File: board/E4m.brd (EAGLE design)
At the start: 49.4 x 100.1 mm, 76 parts, among them IC1 MCP23017SS, Q1 IRL540, Q2 IRL540, Q3 IRL540

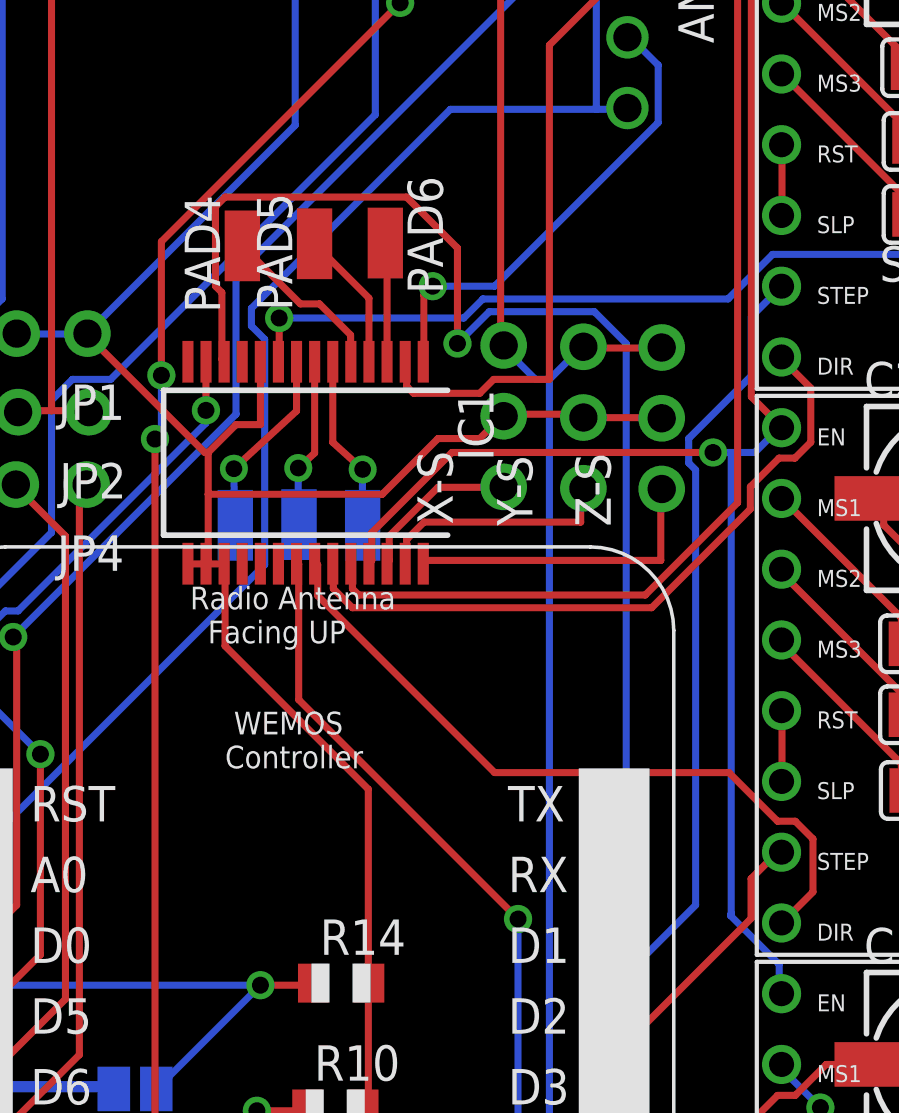
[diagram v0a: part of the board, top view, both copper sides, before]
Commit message: clean clean clean
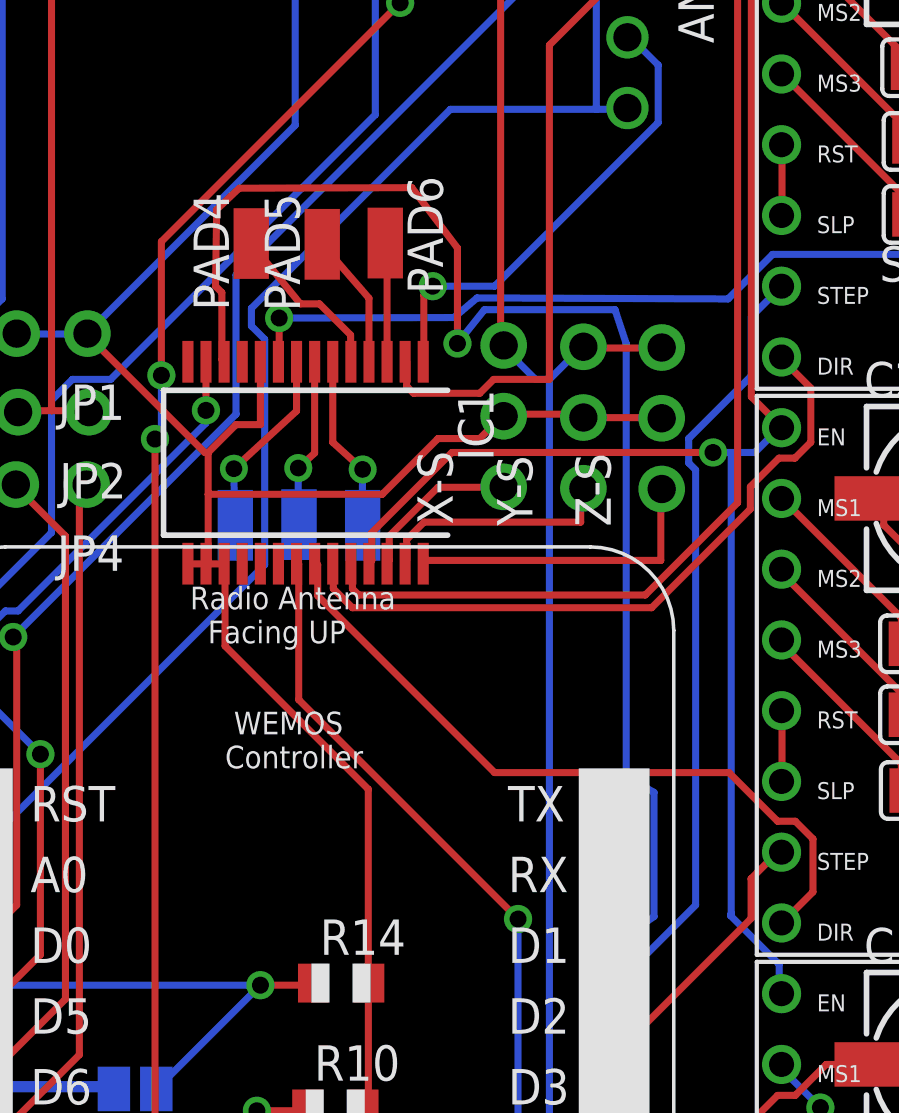
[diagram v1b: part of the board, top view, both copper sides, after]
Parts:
- moved PAD4 0.33 mm to (13.2, 47.3)
- moved PAD5 0.28 mm to (15.7, 47.2)
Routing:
- net SCL: track 48.0 -> 49.5 mm
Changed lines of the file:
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@@
 <element name="PAD2" library="wirepad" package="SMD1,27-2,54" value="WIREPADSMD1,27-254" x="17.1704" y="37.1348" rot="MR0"/>
 <element name="PAD3" library="wirepad" package="SMD1,27-2,54" value="WIREPADSMD1,27-254" x="14.8844" y="37.1602" rot="MR0"/>
-<element name="PAD4" library="wirepad" package="SMD1,27-2,54" value="WIREPADSMD1,27-254" x="12.8524" y="47.1678"/>
-<element name="PAD5" library="wirepad" package="SMD1,27-2,54" value="WIREPADSMD1,27-254" x="15.4432" y="47.244"/>
+<element name="PAD4" library="wirepad" package="SMD1,27-2,54" value="WIREPADSMD1,27-254" x="13.1699" y="47.251621875"/>
+<element name="PAD5" library="wirepad" package="SMD1,27-2,54" value="WIREPADSMD1,27-254" x="15.720059375" y="47.223678125"/>
 <element name="PAD6" library="wirepad" package="SMD1,27-2,54" value="WIREPADSMD1,27-254" x="17.9832" y="47.2694" rot="R180"/>
 <element name="JP3" library="adafruit" package="1X01-CLEANBIG" value="" x="24.0284" y="85.8266"/>
@@
 <wire x1="16.7386" y1="43.9674" x2="15.621" y2="45.085" width="0.254" layer="1"/>
 <wire x1="15.621" y1="45.085" x2="14.9352" y2="45.085" width="0.254" layer="1"/>
-<wire x1="14.9352" y1="45.085" x2="12.8524" y2="47.1678" width="0.254" layer="1"/>
+<wire x1="14.9352" y1="45.085" x2="13.1699" y2="47.251621875" width="0.254" layer="1"/>
 </signal>
 <signal name="N$26" class="3">
 <contactref element="IC1" pad="4"/>
 <contactref element="PAD5" pad="1"/>
-<wire x1="15.4432" y1="47.244" x2="17.397" y2="45.2902" width="0.254" layer="1"/>
+<wire x1="15.720059375" y1="47.223678125" x2="17.397" y2="45.2902" width="0.254" layer="1"/>
 <wire x1="17.397" y1="45.2902" x2="17.397" y2="43.006" width="0.254" layer="1"/>
 </signal>
@@
 <wire x1="12.1158" y1="45.4914" x2="12.1158" y2="43.0911" width="0.254" layer="1"/>
 <wire x1="11.8872" y1="45.72" x2="12.1158" y2="45.4914" width="0.254" layer="1"/>
-<wire x1="11.8872" y1="48.5775" x2="11.8872" y2="45.72" width="0.254" layer="1"/>
-<wire x1="12.2301" y1="48.9204" x2="11.8872" y2="48.5775" width="0.254" layer="1"/>
-<wire x1="18.7452" y1="48.9204" x2="12.2301" y2="48.9204" width="0.254" layer="1"/>
-<wire x1="20.574" y1="47.0916" x2="18.7452" y2="48.9204" width="0.254" layer="1"/>
+<wire x1="11.93038125" y1="48.4733625" x2="11.8872" y2="45.72" width="0.254" layer="1"/>
+<wire x1="12.7381" y1="49.2379" x2="11.93038125" y2="48.4733625" width="0.254" layer="1"/>
+<wire x1="18.9357" y1="49.25821875" x2="12.7381" y2="49.2379" width="0.254" layer="1"/>
+<wire x1="20.574" y1="47.0916" x2="18.9357" y2="49.25821875" width="0.254" layer="1"/>
 <wire x1="20.574" y1="43.6626" x2="20.574" y2="47.0916" width="0.254" layer="1"/>
-<wire x1="21.717" y1="44.8056" x2="20.574" y2="43.6626" width="0.254" layer="16"/>
-<wire x1="25.4889" y1="44.8056" x2="21.717" y2="44.8056" width="0.254" layer="16"/>
-<wire x1="26.6319" y1="43.6626" x2="25.4889" y2="44.8056" width="0.254" layer="16"/>
+<wire x1="21.541740625" y1="44.876721875" x2="20.574" y2="43.6626" width="0.254" layer="16"/>
+<wire x1="26.23058125" y1="44.87671875" x2="21.541740625" y2="44.876721875" width="0.254" layer="16"/>
+<wire x1="26.6319" y1="43.6626" x2="26.23058125" y2="44.87671875" width="0.254" layer="16"/>
 <wire x1="26.6319" y1="28.1178" x2="26.6319" y2="43.6626" width="0.254" layer="16"/>
-<wire x1="27.2034" y1="27.5463" x2="26.6319" y2="28.1178" width="0.254" layer="16"/>
-<wire x1="27.2034" y1="23.0886" x2="27.2034" y2="27.5463" width="0.254" layer="16"/>
-<wire x1="26.289" y1="22.1742" x2="27.2034" y2="23.0886" width="0.254" layer="16"/>
+<wire x1="27.632659375" y1="27.5463" x2="26.6319" y2="28.1178" width="0.254" layer="16"/>
+<wire x1="27.632659375" y1="23.0886" x2="27.632659375" y2="27.5463" width="0.254" layer="16"/>
+<wire x1="26.289" y1="22.1742" x2="27.632659375" y2="23.0886" width="0.254" layer="16"/>
 <wire x1="12.1158" y1="43.0911" x2="12.197" y2="43.006" width="0.254" layer="1"/>
 <wire x1="26.289" y1="22.1742" x2="26.2" y2="22.06" width="0.254" layer="16"/>
@@
 <wire x1="38.2905" y1="50.7492" x2="38.2906" y2="50.9166" width="0.254" layer="1"/>
 <wire x1="14.1732" y1="44.577" x2="14.1732" y2="43.0911" width="0.254" layer="1"/>
-<wire x1="20.8026" y1="44.577" x2="14.1732" y2="44.577" width="0.254" layer="16"/>
-<wire x1="21.4884" y1="45.2628" x2="20.8026" y2="44.577" width="0.254" layer="16"/>
-<wire x1="30.2895" y1="45.2628" x2="21.4884" y2="45.2628" width="0.254" layer="16"/>
+<wire x1="20.449540625" y1="44.59478125" x2="14.1732" y2="44.577" width="0.254" layer="16"/>
+<wire x1="21.27758125" y1="45.298359375" x2="20.449540625" y2="44.59478125" width="0.254" layer="16"/>
+<wire x1="30.2895" y1="45.2628" x2="21.27758125" y2="45.298359375" width="0.254" layer="16"/>
 <wire x1="31.8897" y1="46.863" x2="30.2895" y2="45.2628" width="0.254" layer="16"/>
 <wire x1="43.6626" y1="46.863" x2="38.2905" y2="46.863" width="0.254" layer="16"/>
